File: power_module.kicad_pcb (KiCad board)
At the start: 4 copper layers, 95 x 66 mm, 71 parts, among them J1 USB_C_PD, J2 OUTPUT, J3 I2C_BREAKOUT, Q1 DUAL_N_FET, Q2 DUAL_N_FET, Q3 DUAL_N_FET, Q4 DUAL_N_FET, SW1 ON_OFF, U1 BQ7692003, U2 CH224K, U3 BQ24650, U4 LM5176PWPR

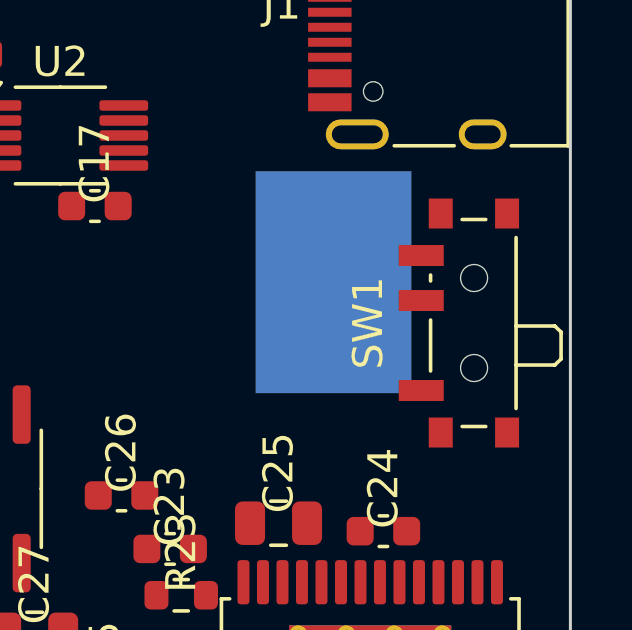
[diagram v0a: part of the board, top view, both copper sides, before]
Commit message: Locked U4
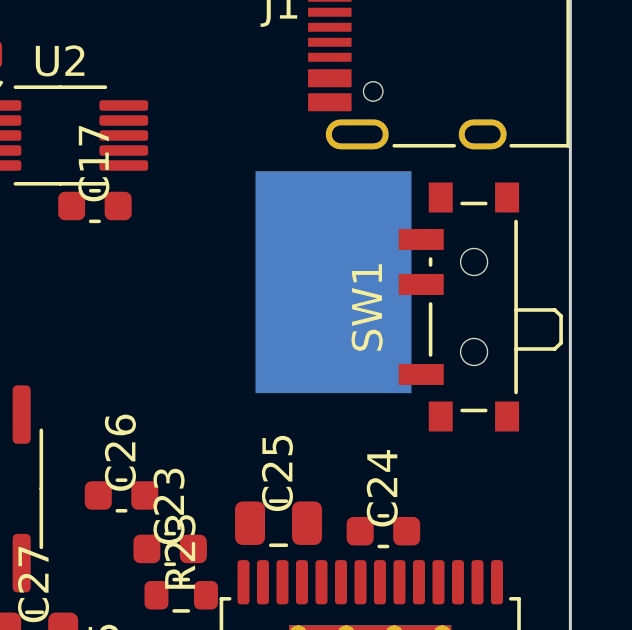
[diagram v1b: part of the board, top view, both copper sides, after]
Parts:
- moved SW1 0.53 mm to (91.5, 31.8)
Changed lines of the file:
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@@
 	(footprint "Button_Switch_SMD:SW_SPDT_PCM12"
 		(layer "F.Cu")
-		(at 91.509276 32.308559 90)
+		(at 91.509276 31.774 90)
 		(descr "Ultraminiature Surface Mount Slide Switch, right-angle, https://www.ckswitches.com/media/1424/pcm.pdf")
 		(property "Reference" "SW1"
@@
 	)
 	(footprint "Package_SO:HTSSOP-28-1EP_4.4x9.7mm_P0.65mm_EP2.85x5.4mm_ThermalVias"
+		(locked yes)
 		(layer "F.Cu")
 		(at 88.377946 43.812013 90)
